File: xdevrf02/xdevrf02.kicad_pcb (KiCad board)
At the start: 4 copper layers, 50.8 x 22.9 mm, 47 parts, among them J1 SWD, P1 USB-C, SW1 RST, SW2 USER, U1 nRF52840, U2 Feather, U3 AP2112K-3.3, U4 LSM6DS3, Y1 32MHz

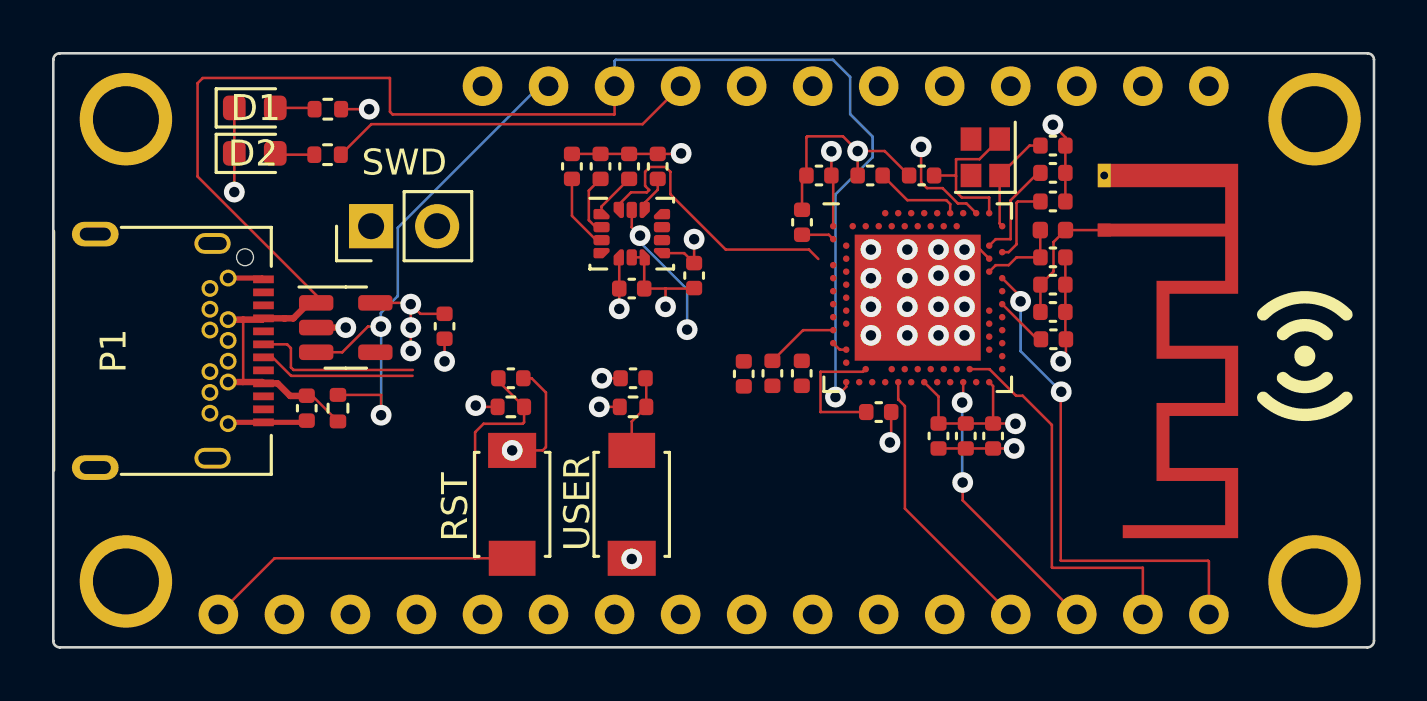
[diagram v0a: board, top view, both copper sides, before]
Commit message: design rules
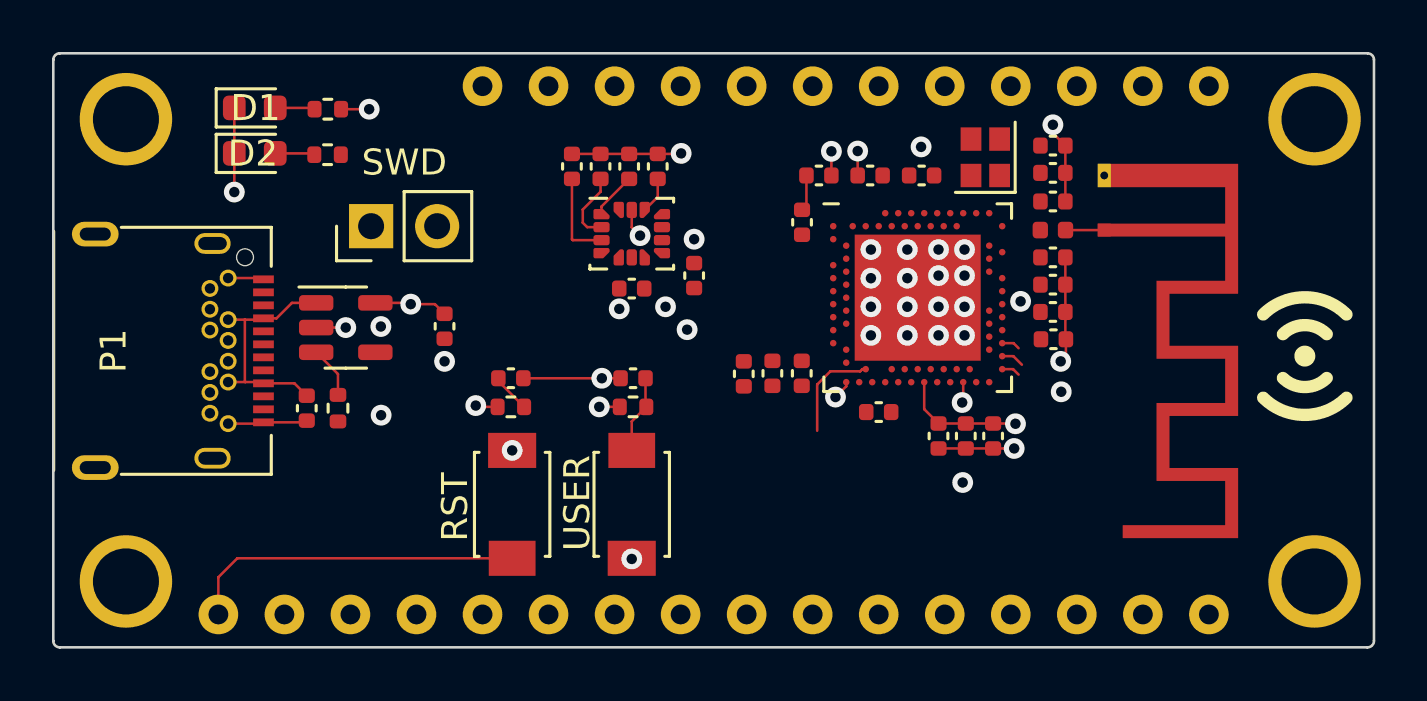
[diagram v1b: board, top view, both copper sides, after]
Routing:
- net VBUS: track 64.7 -> 10.0 mm
- net /d2: track 19.7 -> 0.00 mm
- net /enable: track 20.9 -> 1.99 mm
- net GND: track 40.3 -> 25.1 mm, vias 28 -> 27
- net /serial_tx: track 14.8 -> 0.00 mm
- net VDD: track 30.0 -> 15.5 mm, vias 12 -> 10
- net /d13: track 14.2 -> 0.00 mm
- net /sda: track 13.9 -> 0.00 mm
- net /miso: track 10.7 -> 0.00 mm
- net /serial_rx: track 11.2 -> 0.80 mm
- net /nreset: track 21.2 -> 14.5 mm
- net Net-(P1-PadA6): track 6.59 -> 0.00 mm
- net Net-(C17-Pad1): track 6.07 -> 0.00 mm
- net Net-(P1-PadA7): track 6.03 -> 0.00 mm
- net /scl: track 5.49 -> 1.12 mm
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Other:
- rule pad_to_mask_clearance: 0 -> 0.05
